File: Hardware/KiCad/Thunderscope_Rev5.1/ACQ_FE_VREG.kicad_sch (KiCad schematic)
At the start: 63 parts, among them U13 LM27761, U14 TPS7A9101, U15 TPS7A9101, U16 TPS7A2033, U9 TPS7A2033

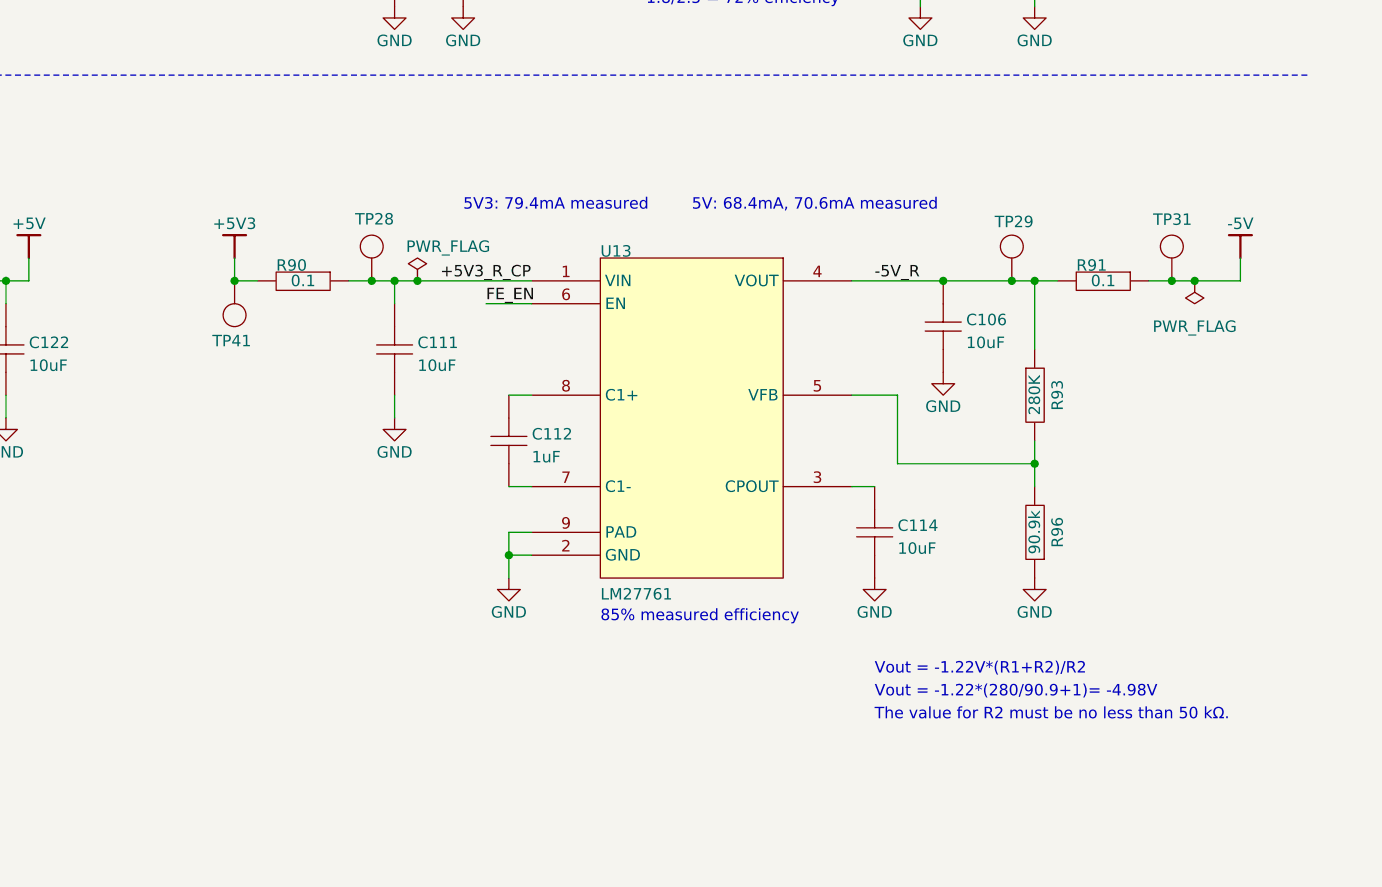
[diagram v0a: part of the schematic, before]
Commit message: Added Charge Pump Output Filter as per #335
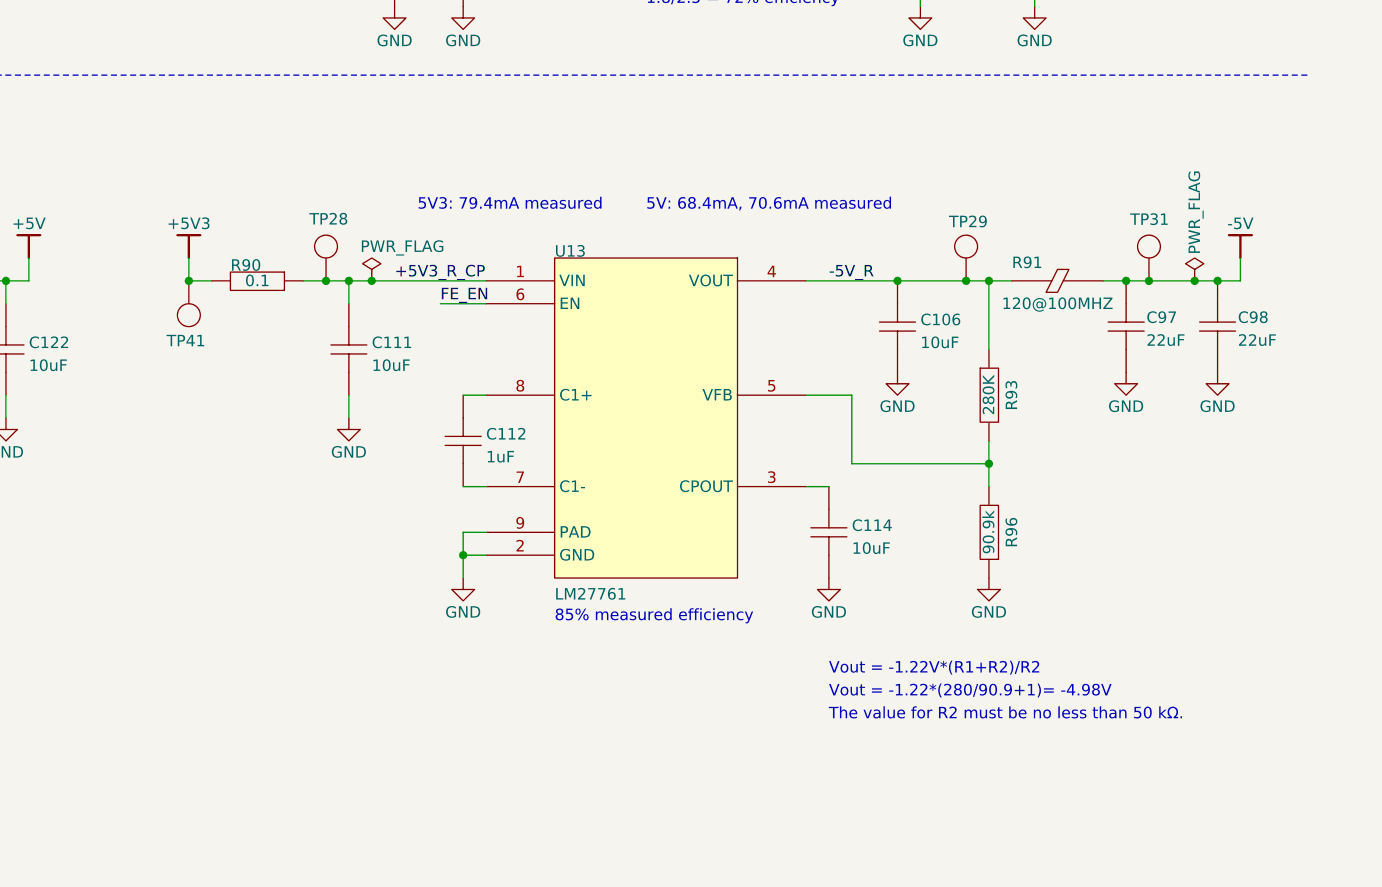
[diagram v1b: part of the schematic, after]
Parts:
- added C97, C98: 22uF, Thunderscope_Rev5:GEN_C_0805, symbol Thunderscope_Rev5:CAP 22uF 25V X5R 0805
- R91: value 0.1 -> 120@100MHZ; symbol Thunderscope_Rev5:RES 0.1 OHM 1% 1/6W 0402 -> Thunderscope_Rev5:FERRITE BEAD 120 OHM 0402; HOUSE PART NUMBER (none) -> BLM15PX121SN1D; MANUFACTURER Panasonic -> Murata; MANUFACTURER PART NUMBER ERJ-2BSFR10X -> BLM15PX121SN1D; SUPPLIER PART NUMBER 1 667-ERJ-2BSFR10X -> 81-BLM15PX121SN1D
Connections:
- net -5V: now also C97.2, C98.2
- net GND: now also C97.1, C98.1
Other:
- moved on the sheet: C106, C111, C112, C114, R90, R91, R93, R96, TP28, TP29, TP31, TP41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

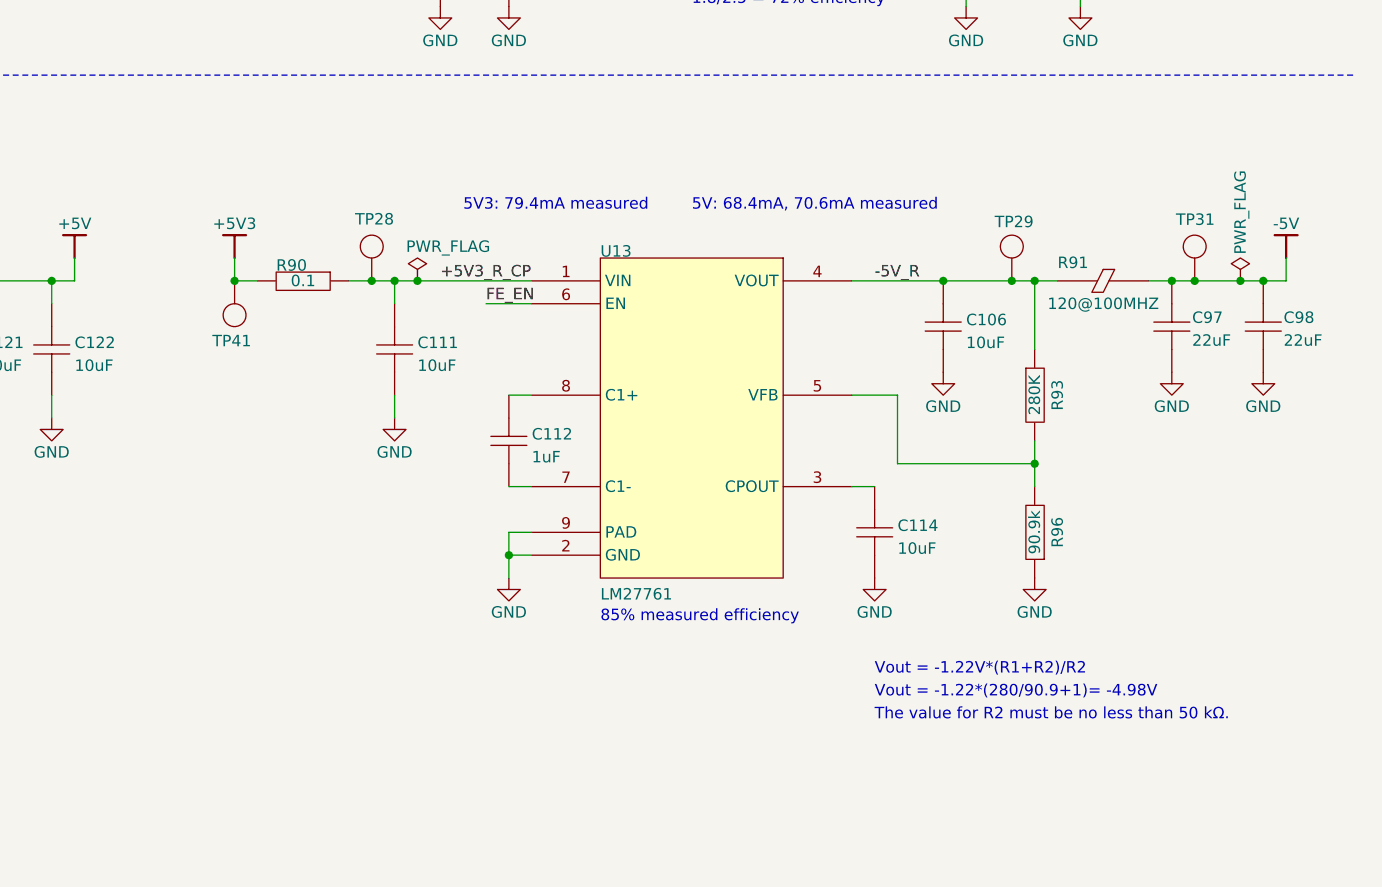
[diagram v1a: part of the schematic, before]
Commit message: Added 1uF at -5V output as per #354
Also added net label to +VUSB PG output
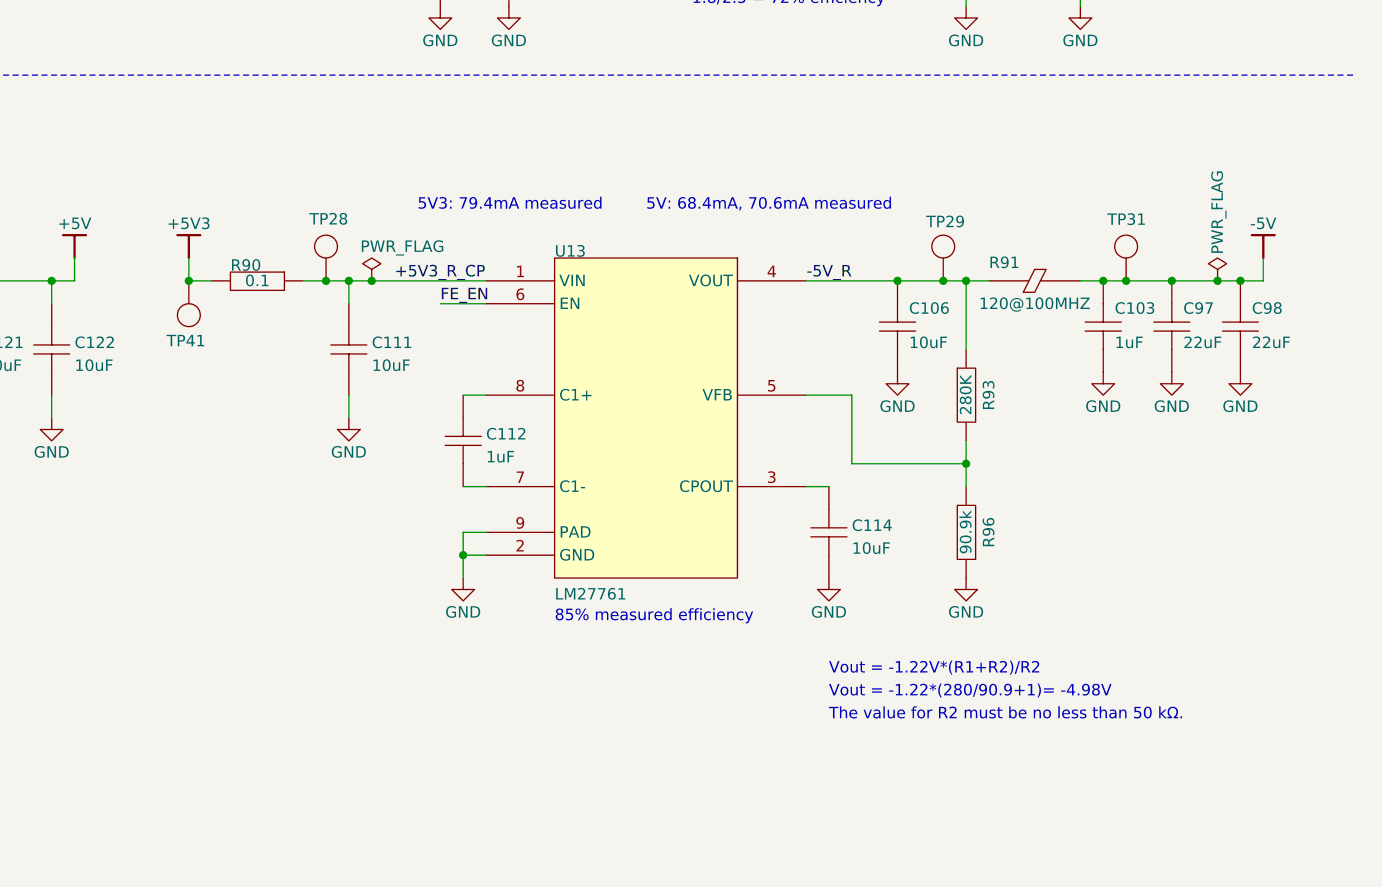
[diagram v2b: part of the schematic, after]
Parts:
- added C103: 1uF, Thunderscope_Rev5:GEN_C_0402, symbol Thunderscope_Rev5:CAP 1uF 25V X5R 0402
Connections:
- net -5V: now also C103.1
- net GND: now also C103.2
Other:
- moved on the sheet: C106, C111, C112, C114, C98, R90, R91, R93, R96, TP28, TP29, TP31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
